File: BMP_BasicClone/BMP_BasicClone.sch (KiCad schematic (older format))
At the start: 55 parts, among them J1 BARREL_JACK, J2 CONN_02X06, J3 CONN_02X06, Q1 MMBT3904, Q2 MMBT3904, Q3 MMBT3904, Q4 MMBT3904

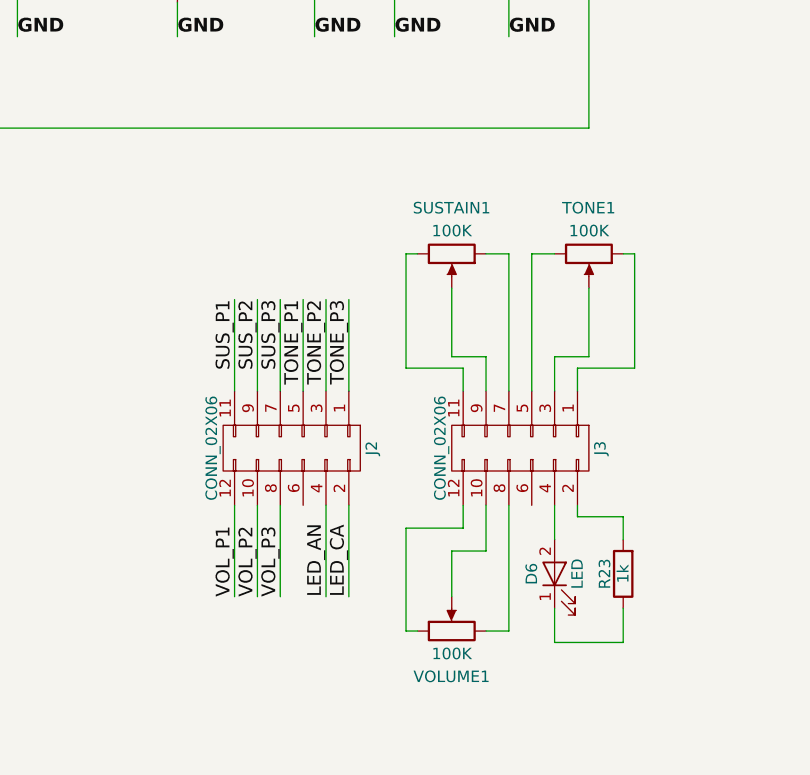
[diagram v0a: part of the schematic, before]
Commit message: Update
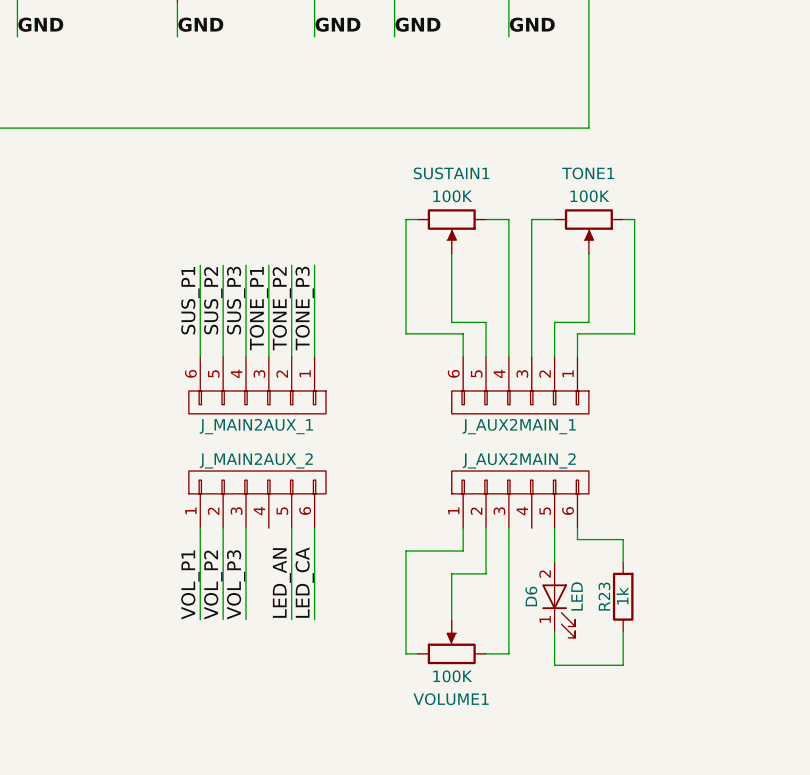
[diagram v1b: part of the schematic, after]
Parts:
- removed J2, J3: CONN_02X06, Pin_Headers:Pin_Header_Straight_2x06_Pitch2.54mm, symbol CONN_02X06
- added J_AUX2MAIN_1, J_AUX2MAIN_2, J_MAIN2AUX_1, J_MAIN2AUX_2: CONN_01X06, Pin_Headers:Pin_Header_Straight_1x06_Pitch2.54mm, symbol CONN_01X06
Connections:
- net GND: now also J_MAIN2AUX_2.3 (P3), J_MAIN2AUX_2.6 (P6)
- net LED_AN: now also J_MAIN2AUX_2.5 (P5)
- net SUS_P1: now also J_MAIN2AUX_1.6 (P6)
- net SUS_P2: now also J_MAIN2AUX_1.5 (P5)
- net SUS_P3: now also J_MAIN2AUX_1.4 (P4)
- net TONE_P1: now also J_MAIN2AUX_1.3 (P3)
- net TONE_P2: now also J_MAIN2AUX_1.2 (P2)
- net TONE_P3: now also J_MAIN2AUX_1.1 (P1)
- net VOL_P1: now also J_MAIN2AUX_2.1 (P1)
- net VOL_P2: now also J_MAIN2AUX_2.2 (P2)
- net at D6.2 (A): now also J_AUX2MAIN_2.5 (P5)
- net at R23.2: now also J_AUX2MAIN_2.6 (P6)
- net at TONE1.1: now also J_AUX2MAIN_1.1 (P1)
- net at VOLUME1.2: now also J_AUX2MAIN_2.2 (P2)
- net at SUSTAIN1.3: now also J_AUX2MAIN_1.6 (P6)
- net at VOLUME1.1: now also J_AUX2MAIN_2.1 (P1)
- net at TONE1.2: now also J_AUX2MAIN_1.2 (P2)
- net at TONE1.3: now also J_AUX2MAIN_1.3 (P3)
- net at SUSTAIN1.1: now also J_AUX2MAIN_1.4 (P4)
- net at VOLUME1.3: now also J_AUX2MAIN_2.3 (P3)
- net at SUSTAIN1.2: now also J_AUX2MAIN_1.5 (P5)
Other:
- moved on the sheet: D6, R23, SUSTAIN1, TONE1, VOLUME1
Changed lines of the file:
@@
 L LED D6
 U 1 1 5A2E0726
-P 9200 5750
-F 0 "D6" H 9200 5850 50  0000 C CNN
-F 1 "LED" H 9200 5650 50  0000 C CNN
-F 2 "LEDs:LED_D5.0mm" H 9200 5750 50  0001 C CNN
-F 3 "" H 9200 5750 50  0001 C CNN
-	1    9200 5750
+P 9200 5850
+F 0 "D6" H 9200 5950 50  0000 C CNN
+F 1 "LED" H 9200 5750 50  0000 C CNN
+F 2 "LEDs:LED_D5.0mm" H 9200 5850 50  0001 C CNN
+F 3 "" H 9200 5850 50  0001 C CNN
+	1    9200 5850
 	0    -1   -1   0
 $EndComp
@@
 L R R23
 U 1 1 5A2E81A3
-P 9500 5750
-F 0 "R23" V 9580 5750 50  0000 C CNN
-F 1 "1k" V 9500 5750 50  0000 C CNN
-F 2 "Resistors_SMD:R_0805" V 9430 5750 50  0001 C CNN
-F 3 "" H 9500 5750 50  0001 C CNN
-	1    9500 5750
+P 9500 5850
+F 0 "R23" V 9580 5850 50  0000 C CNN
+F 1 "1k" V 9500 5850 50  0000 C CNN
+F 2 "Resistors_SMD:R_0805" V 9430 5850 50  0001 C CNN
+F 3 "" H 9500 5850 50  0001 C CNN
+	1    9500 5850
 	-1   0    0    1
 $EndComp
@@
 $EndComp
 $Comp
-L CONN_02X06 J3
-U 1 1 5A33F471
-P 9050 5200
-F 0 "J3" H 9050 5550 50  0000 C CNN
-F 1 "CONN_02X06" H 9050 4850 50  0000 C CNN
-F 2 "Pin_Headers:Pin_Header_Straight_2x06_Pitch2.54mm" H 9050 4000 50  0001 C CNN
-F 3 "" H 9050 4000 50  0001 C CNN
-	1    9050 5200
-	0    1    1    0
-$EndComp
-$Comp
 L POT SUSTAIN1
 U 1 1 5A34007A
-P 8750 4350
-F 0 "SUSTAIN1" V 8550 4350 50  0000 C CNN
-F 1 "100K" V 8650 4350 50  0000 C CNN
-F 2 "Potentiometers:Potentiometer_Bourns_PTV09A-1_Horizontal" H 8750 4350 50  0001 C CNN
-F 3 "" H 8750 4350 50  0001 C CNN
-	1    8750 4350
+P 8750 4200
+F 0 "SUSTAIN1" V 8550 4200 50  0000 C CNN
+F 1 "100K" V 8650 4200 50  0000 C CNN
+F 2 "Potentiometers:Potentiometer_Bourns_PTV09A-1_Horizontal" H 8750 4200 50  0001 C CNN
+F 3 "" H 8750 4200 50  0001 C CNN
+	1    8750 4200
 	0    1    1    0
 $EndComp
@@
 Text Label 4250 5400 1    60   ~ 0
 SUS_P2
-$Comp
-L CONN_02X06 J2
-U 1 1 5A342A65
-P 8050 5200
-F 0 "J2" H 8050 5550 50  0000 C CNN
-F 1 "CONN_02X06" H 8050 4850 50  0000 C CNN
-F 2 "Pin_Headers:Pin_Header_Straight_2x06_Pitch2.54mm" H 8050 4000 50  0001 C CNN
-F 3 "" H 8050 4000 50  0001 C CNN
-	1    8050 5200
-	0    1    1    0
-$EndComp
-Text Label 7800 4550 3    60   ~ 0
+Text Label 7650 4400 3    60   ~ 0
 SUS_P1
-Text Label 7900 4550 3    60   ~ 0
+Text Label 7750 4400 3    60   ~ 0
 SUS_P2
-Text Label 8000 4550 3    60   ~ 0
+Text Label 7850 4400 3    60   ~ 0
 SUS_P3
 $Comp
 L POT TONE1
 U 1 1 5A3434FD
-P 9350 4350
-F 0 "TONE1" V 9150 4350 50  0000 C CNN
-F 1 "100K" V 9250 4350 50  0000 C CNN
-F 2 "Potentiometers:Potentiometer_Bourns_PTV09A-1_Horizontal" H 9350 4350 50  0001 C CNN
-F 3 "" H 9350 4350 50  0001 C CNN
-	1    9350 4350
+P 9350 4200
+F 0 "TONE1" V 9150 4200 50  0000 C CNN
+F 1 "100K" V 9250 4200 50  0000 C CNN
+F 2 "Potentiometers:Potentiometer_Bourns_PTV09A-1_Horizontal" H 9350 4200 50  0001 C CNN
+F 3 "" H 9350 4200 50  0001 C CNN
+	1    9350 4200
 	0    1    1    0
 $EndComp
-Text Label 8100 4550 3    60   ~ 0
+Text Label 7950 4400 3    60   ~ 0
 TONE_P1
-Text Label 8200 4550 3    60   ~ 0
+Text Label 8050 4400 3    60   ~ 0
 TONE_P2
-Text Label 8300 4550 3    60   ~ 0
+Text Label 8150 4400 3    60   ~ 0
 TONE_P3
 Text Label 7550 2400 3    60   ~ 0
@@
 Text Label 7400 2250 0    60   ~ 0
 TONE_P2
-Text Label 7800 5850 1    60   ~ 0
+Text Label 7650 5950 1    60   ~ 0
 VOL_P1
-Text Label 7900 5850 1    60   ~ 0
+Text Label 7750 5950 1    60   ~ 0
 VOL_P2
-Text Label 8000 5850 1    60   ~ 0
+Text Label 7850 5950 1    60   ~ 0
 VOL_P3
-Text Label 8200 5850 1    60   ~ 0
+Text Label 8050 5950 1    60   ~ 0
 LED_AN
-Text Label 8300 5850 1    60   ~ 0
+Text Label 8150 5950 1    60   ~ 0
 LED_CA
 $Comp
 L POT VOLUME1
 U 1 1 5A346136
-P 8750 6000
-F 0 "VOLUME1" V 8550 6000 50  0000 C CNN
-F 1 "100K" V 8650 6000 50  0000 C CNN
-F 2 "Potentiometers:Potentiometer_Bourns_PTV09A-1_Horizontal" H 8750 6000 50  0001 C CNN
-F 3 "" H 8750 6000 50  0001 C CNN
-	1    8750 6000
+P 8750 6100
+F 0 "VOLUME1" V 8550 6100 50  0000 C CNN
+F 1 "100K" V 8650 6100 50  0000 C CNN
+F 2 "Potentiometers:Potentiometer_Bourns_PTV09A-1_Horizontal" H 8750 6100 50  0001 C CNN
+F 3 "" H 8750 6100 50  0001 C CNN
+	1    8750 6100
 	0    -1   -1   0
 $EndComp
@@
 VOL_P3
 Wire Wire Line
-	9300 5500 9300 5450
-Wire Wire Line
-	9500 5500 9300 5500
-Wire Wire Line
-	9500 5600 9500 5500
-Wire Wire Line
-	9500 6050 9500 5900
-Wire Wire Line
-	9200 6050 9500 6050
-Wire Wire Line
-	9200 5900 9200 6050
-Wire Wire Line
-	9200 5600 9200 5450
-Wire Wire Line
-	8800 5550 8800 5450
-Wire Wire Line
-	8550 5550 8800 5550
-Wire Wire Line
-	8550 6000 8550 5550
-Wire Wire Line
-	8600 6000 8550 6000
-Wire Wire Line
-	8900 5650 8900 5450
-Wire Wire Line
-	8750 5650 8900 5650
-Wire Wire Line
-	8750 5850 8750 5650
-Wire Wire Line
-	9000 6000 9000 5450
-Wire Wire Line
-	8900 6000 9000 6000
-Wire Wire Line
-	8200 5450 8200 5850
-Wire Wire Line
-	8300 5450 8300 5850
-Wire Wire Line
-	8000 5450 8000 5850
-Wire Wire Line
-	7900 5450 7900 5850
-Wire Wire Line
-	7800 5450 7800 5850
-Wire Wire Line
-	8300 4950 8300 4550
-Wire Wire Line
-	8200 4550 8200 4950
-Wire Wire Line
-	8100 4550 8100 4950
-Wire Wire Line
-	9550 4350 9500 4350
-Wire Wire Line
-	9550 4850 9550 4350
-Wire Wire Line
-	9300 4850 9550 4850
-Wire Wire Line
-	9300 4950 9300 4850
-Wire Wire Line
-	9200 4800 9200 4950
-Wire Wire Line
-	9350 4800 9200 4800
-Wire Wire Line
-	9350 4500 9350 4800
-Wire Wire Line
-	9100 4350 9100 4950
-Wire Wire Line
-	9200 4350 9100 4350
-Wire Wire Line
-	8000 4950 8000 4550
-Wire Wire Line
-	7900 4550 7900 4950
-Wire Wire Line
-	7800 4950 7800 4550
-Wire Wire Line
-	8900 4800 8750 4800
-Wire Wire Line
-	8900 4950 8900 4800
-Wire Wire Line
-	8750 4800 8750 4500
-Wire Wire Line
-	8550 4350 8600 4350
-Wire Wire Line
-	8550 4850 8550 4350
-Wire Wire Line
-	8800 4850 8550 4850
-Wire Wire Line
-	8800 4950 8800 4850
-Wire Wire Line
-	9000 4350 9000 4950
-Wire Wire Line
-	8900 4350 9000 4350
+	9300 5600 9300 5550
+Wire Wire Line
+	9500 5600 9300 5600
+Wire Wire Line
+	9500 5700 9500 5600
+Wire Wire Line
+	9500 6150 9500 6000
+Wire Wire Line
+	9200 6150 9500 6150
+Wire Wire Line
+	9200 6000 9200 6150
+Wire Wire Line
+	9200 5700 9200 5550
+Wire Wire Line
+	8800 5650 8800 5550
+Wire Wire Line
+	8550 5650 8800 5650
+Wire Wire Line
+	8550 6100 8550 5650
+Wire Wire Line
+	8600 6100 8550 6100
+Wire Wire Line
+	8900 5750 8900 5550
+Wire Wire Line
+	8750 5750 8900 5750
+Wire Wire Line
+	8750 5950 8750 5750
+Wire Wire Line
+	9000 6100 9000 5550
+Wire Wire Line
+	8900 6100 9000 6100
+Wire Wire Line
+	8050 5550 8050 5950
+Wire Wire Line
+	8150 5550 8150 5950
+Wire Wire Line
+	7850 5550 7850 5950
+Wire Wire Line
+	7750 5550 7750 5950
+Wire Wire Line
+	7650 5550 7650 5950
+Wire Wire Line
+	8150 4800 8150 4400
+Wire Wire Line
+	8050 4400 8050 4800
+Wire Wire Line
+	7950 4400 7950 4800
+Wire Wire Line
+	9550 4200 9500 4200
+Wire Wire Line
+	9550 4700 9550 4200
+Wire Wire Line
+	9300 4700 9550 4700
+Wire Wire Line
+	9300 4800 9300 4700
+Wire Wire Line
+	9200 4650 9200 4800
+Wire Wire Line
+	9350 4650 9200 4650
+Wire Wire Line
+	9350 4350 9350 4650
+Wire Wire Line
+	9100 4200 9100 4800
+Wire Wire Line
+	9200 4200 9100 4200
+Wire Wire Line
+	7850 4800 7850 4400
+Wire Wire Line
+	7750 4400 7750 4800
+Wire Wire Line
+	7650 4800 7650 4400
+Wire Wire Line
+	8900 4650 8750 4650
+Wire Wire Line
+	8900 4800 8900 4650
+Wire Wire Line
+	8750 4650 8750 4350
+Wire Wire Line
+	8550 4200 8600 4200
+Wire Wire Line
+	8550 4700 8550 4200
+Wire Wire Line
+	8800 4700 8550 4700
+Wire Wire Line
+	8800 4800 8800 4700
+Wire Wire Line
+	9000 4200 9000 4800
+Wire Wire Line
+	8900 4200 9000 4200
 Connection ~ 6850 1950
 Wire Wire Line
@@
 Wire Wire Line
 	6300 3800 6300 6550
+$Comp
+L CONN_01X06 J_MAIN2AUX_1
+U 1 1 5A3EEED2
+P 7900 5000
+F 0 "J_MAIN2AUX_1" V 8000 5000 50  0000 C CNN
+F 1 "CONN_01X06" V 8000 5000 50  0001 C CNN
+F 2 "Pin_Headers:Pin_Header_Straight_1x06_Pitch2.54mm" H 7900 5000 50  0001 C CNN
+F 3 "" H 7900 5000 50  0001 C CNN
+	1    7900 5000
+	0    1    1    0
+$EndComp
+$Comp
+L CONN_01X06 J_MAIN2AUX_2
+U 1 1 5A3EEFA8
+P 7900 5350
+F 0 "J_MAIN2AUX_2" V 8000 5350 50  0000 C CNN
+F 1 "CONN_01X06" V 8000 5350 50  0001 C CNN
+F 2 "Pin_Headers:Pin_Header_Straight_1x06_Pitch2.54mm" H 7900 5350 50  0001 C CNN
+F 3 "" H 7900 5350 50  0001 C CNN
+	1    7900 5350
+	0    -1   -1   0
+$EndComp
+$Comp
+L CONN_01X06 J_AUX2MAIN_1
+U 1 1 5A3F0090
+P 9050 5000
+F 0 "J_AUX2MAIN_1" V 9150 5000 50  0000 C CNN
+F 1 "CONN_01X06" V 9150 5000 50  0001 C CNN
+F 2 "Pin_Headers:Pin_Header_Straight_1x06_Pitch2.54mm" H 9050 5000 50  0001 C CNN
+F 3 "" H 9050 5000 50  0001 C CNN
+	1    9050 5000
+	0    1    1    0
+$EndComp
+$Comp
+L CONN_01X06 J_AUX2MAIN_2
+U 1 1 5A3F0164
+P 9050 5350
+F 0 "J_AUX2MAIN_2" V 9150 5350 50  0000 C CNN
+F 1 "CONN_01X06" V 9150 5350 50  0001 C CNN
+F 2 "Pin_Headers:Pin_Header_Straight_1x06_Pitch2.54mm" H 9050 5350 50  0001 C CNN
+F 3 "" H 9050 5350 50  0001 C CNN
+	1    9050 5350
+	0    -1   -1   0
+$EndComp
 $EndSCHEMATC
